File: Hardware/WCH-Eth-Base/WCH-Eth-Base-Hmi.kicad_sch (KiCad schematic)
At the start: 1 part, among them SW3 RotaryEncoder_Switch

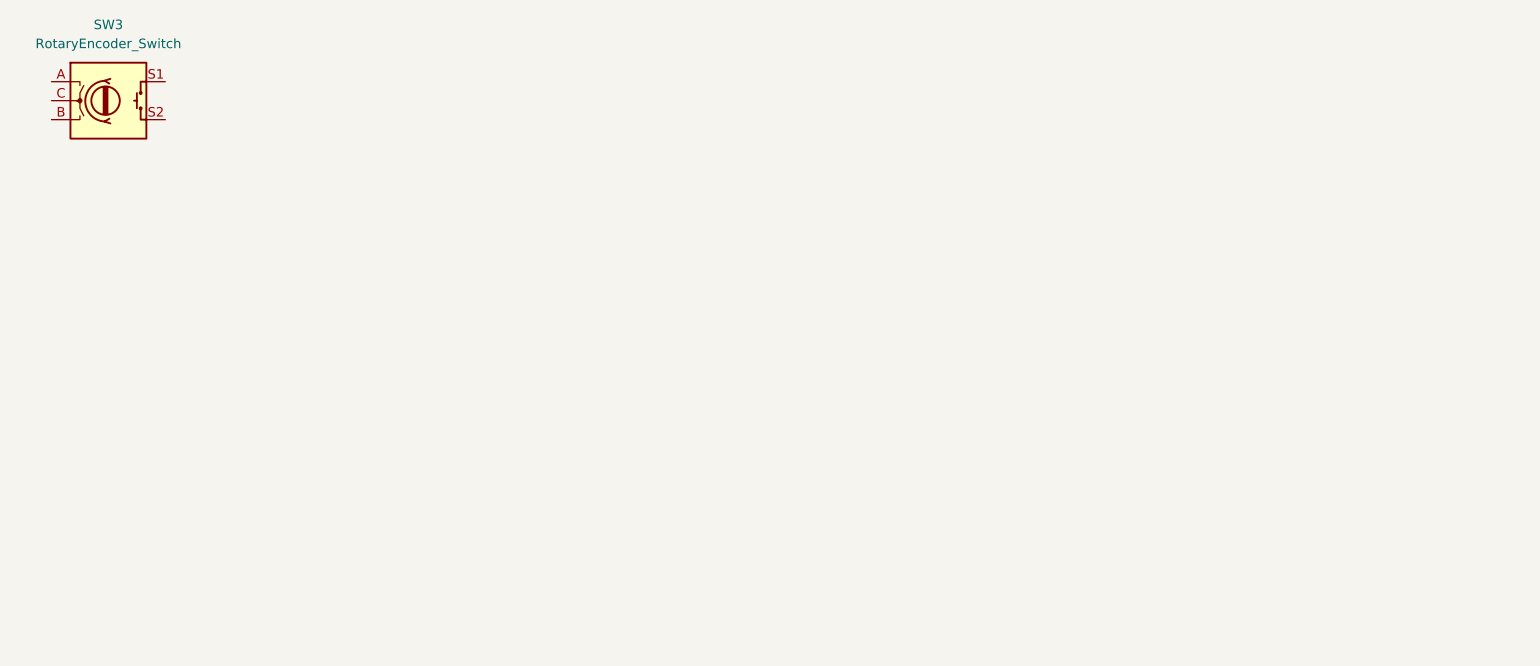
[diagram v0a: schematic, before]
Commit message: add Files and First Layout things
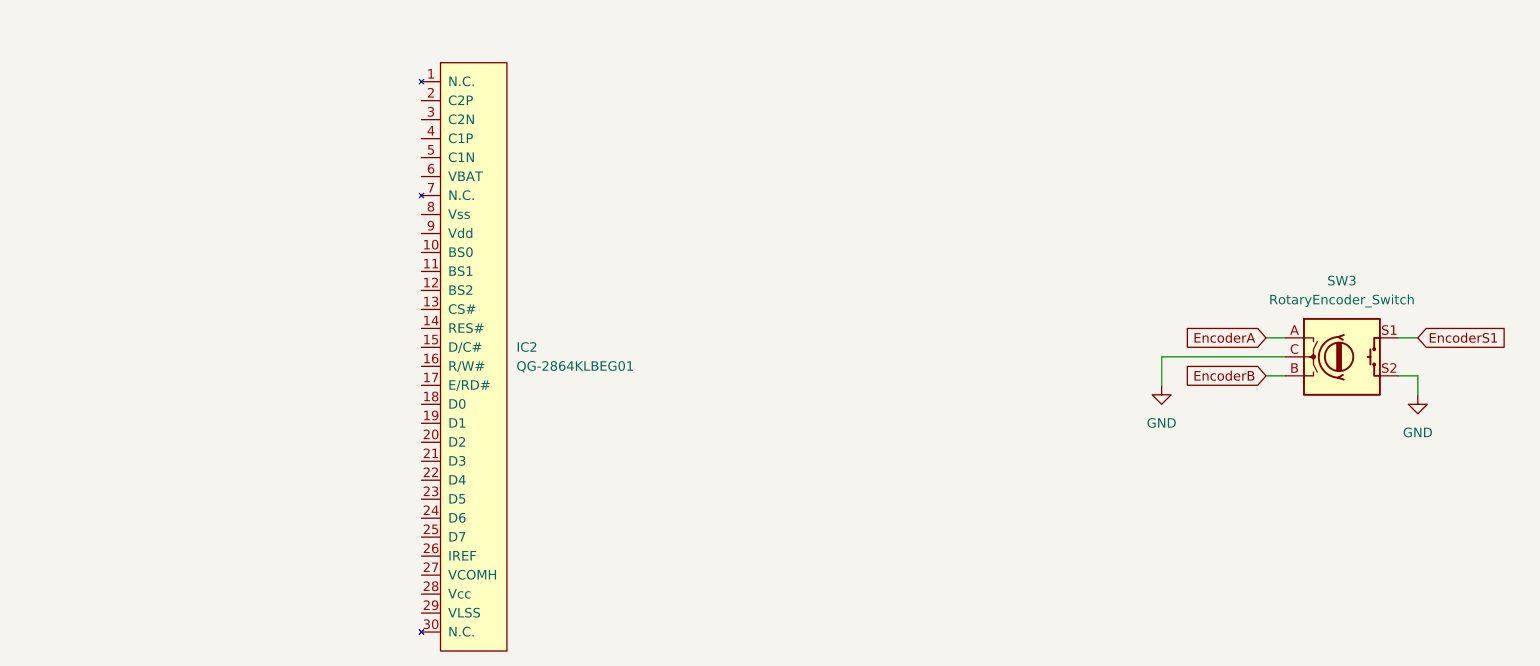
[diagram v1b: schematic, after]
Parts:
- added IC2: QG-2864KLBEG01, symbol Techbeard:QG-2864KLBEG01
- SW3: footprint Rotary_Encoder:RotaryEncoder_Alps_EC11E-Switch_Vertical_H20mm_CircularMountingHoles -> Techbeard:STEC11B09
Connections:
- net EncoderA: now reaches SW3.A
- net EncoderB: now reaches SW3.B
- net GND: now reaches SW3.C
- net GND: now also SW3.S2
- net EncoderS1: now reaches SW3.S1
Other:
- moved on the sheet: SW3
